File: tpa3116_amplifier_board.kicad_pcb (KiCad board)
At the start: 2 copper layers, 61.6 x 50.8 mm, 41 parts, among them IC1 TPA3116D2QDADRQ1, J1 power_supply, J2 Conn_01x04, J3 power_supply, J4 output_right

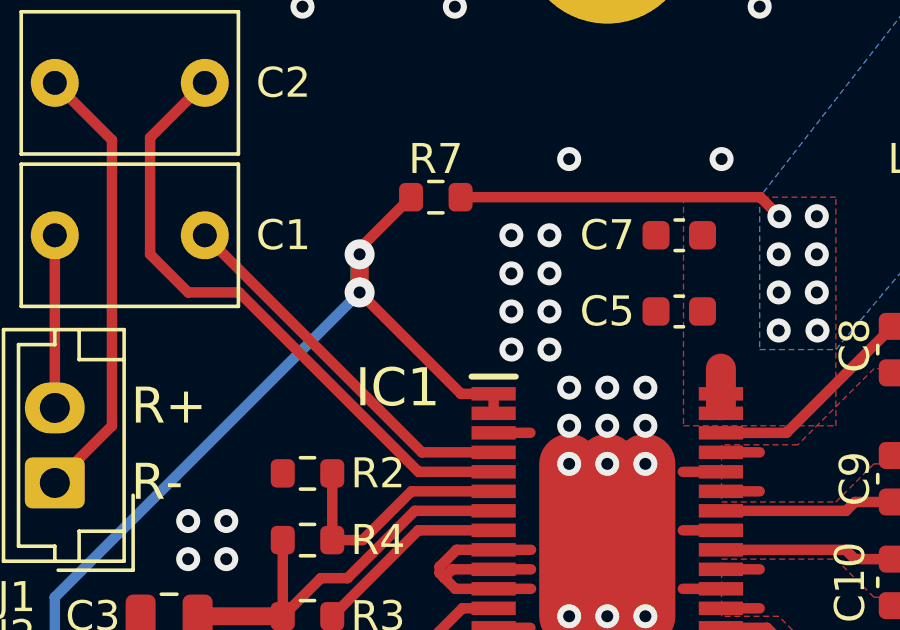
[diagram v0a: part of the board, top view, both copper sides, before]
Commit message: исправил ошибку в схеме
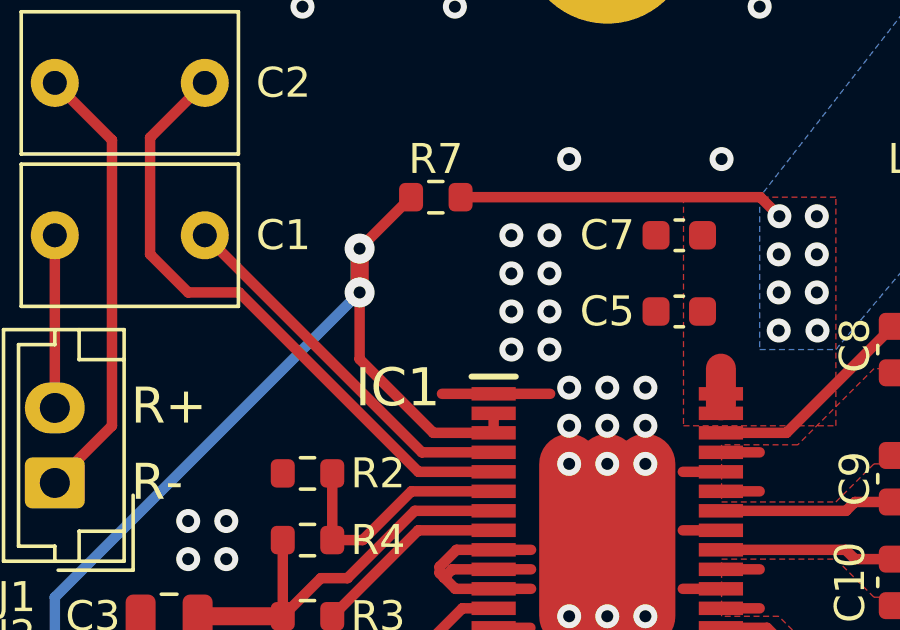
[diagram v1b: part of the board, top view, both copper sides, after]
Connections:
- IC1 pad 1: /SD_LR -> GND
- IC1 pad 3: GND -> /SD_LR
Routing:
- net GND: track 38.0 -> 40.4 mm
- net /SD_LR: track 31.2 -> 33.2 mm
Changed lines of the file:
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@@
       (stroke (width 0.1) (type solid)) (layer "F.Fab"))
     (pad "1" smd rect (at -3.788 -4.875 90) (size 0.45 1.475) (layers "F.Cu" "F.Paste" "F.Mask")
-      (net 16 "/SD_LR") (pinfunction "MODSEL") (pintype "passive"))
+      (net 5 "GND") (pinfunction "MODSEL") (pintype "passive"))
     (pad "2" smd rect (at -3.788 -4.225 90) (size 0.45 1.475) (layers "F.Cu" "F.Paste" "F.Mask")
       (net 16 "/SD_LR") (pinfunction "SD") (pintype "passive"))
     (pad "3" smd rect (at -3.788 -3.575 90) (size 0.45 1.475) (layers "F.Cu" "F.Paste" "F.Mask")
-      (net 5 "GND") (pinfunction "FAULT") (pintype "passive"))
+      (net 16 "/SD_LR") (pinfunction "FAULT") (pintype "passive"))
     (pad "4" smd rect (at -3.788 -2.925 90) (size 0.45 1.475) (layers "F.Cu" "F.Paste" "F.Mask")
       (net 2 "Net-(IC1-RINP)") (pinfunction "RINP") (pintype "passive"))
@@
   (segment (start 128.248 121.64) (end 126.978 121.64) (width 0.35) (layer "F.Cu") (net 5))
   (segment (start 120.672 124.24) (end 121.898 124.24) (width 0.35) (layer "F.Cu") (net 5))
-  (segment (start 120.672 116.44) (end 121.898 116.44) (width 0.35) (layer "F.Cu") (net 5))
   (segment (start 120.672 121.64) (end 121.92 121.64) (width 0.35) (layer "F.Cu") (net 5))
   (segment (start 120.672 120.34) (end 121.92 120.34) (width 0.35) (layer "F.Cu") (net 5))
   (segment (start 128.248 117.74) (end 126.978 117.74) (width 0.35) (layer "F.Cu") (net 5))
+  (segment (start 122.555 115.14) (end 118.95 115.14) (width 0.35) (layer "F.Cu") (net 5))
   (segment (start 119.294 120.99) (end 120.672 120.99) (width 0.35) (layer "F.Cu") (net 5))
   (segment (start 120.672 123.59) (end 121.898 123.59) (width 0.35) (layer "F.Cu") (net 5))
@@
   (segment (start 129.785 122.94) (end 133.985 127.14) (width 0.35) (layer "F.Cu") (net 15))
   (segment (start 128.248 122.94) (end 129.785 122.94) (width 0.35) (layer "F.Cu") (net 15))
-  (segment (start 119.585 115.14) (end 120.672 115.14) (width 0.35) (layer "F.Cu") (net 16))
-  (segment (start 116.205 110.3) (end 116.205 110.49) (width 0.35) (layer "F.Cu") (net 16))
-  (segment (start 120.672 115.79) (end 120.672 115.14) (width 0.35) (layer "F.Cu") (net 16))
-  (segment (start 116.205 111.76) (end 119.585 115.14) (width 0.35) (layer "F.Cu") (net 16))
-  (segment (start 116.205 110.49) (end 116.205 111.76) (width 0.6) (layer "F.Cu") (net 16))
-  (segment (start 117.92 108.585) (end 116.205 110.3) (width 0.35) (layer "F.Cu") (net 16))
-  (via (at 116.205 110.49) (size 1) (drill 0.4) (layers "F.Cu" "B.Cu") (net 16))
+  (segment (start 118.6625 116.44) (end 120.672 116.44) (width 0.35) (layer "F.Cu") (net 16))
+  (segment (start 116.205 110.3) (end 117.92 108.585) (width 0.35) (layer "F.Cu") (net 16))
+  (segment (start 120.672 116.44) (end 120.672 115.79) (width 0.35) (layer "F.Cu") (net 16))
+  (segment (start 116.205 111.76) (end 116.205 113.9825) (width 0.35) (layer "F.Cu") (net 16))
+  (segment (start 116.205 113.9825) (end 118.6625 116.44) (width 0.35) (layer "F.Cu") (net 16))
+  (segment (start 116.205 110.3) (end 116.205 111.76) (width 0.6) (layer "F.Cu") (net 16))
+  (via (at 116.205 110.3) (size 1) (drill 0.4) (layers "F.Cu" "B.Cu") (net 16))
   (via (at 116.205 111.76) (size 1) (drill 0.4) (layers "F.Cu" "B.Cu") (net 16))
+  (segment (start 106.045 121.92) (end 106.045 127.04) (width 0.35) (layer "B.Cu") (net 16))
+  (segment (start 116.205 110.3) (end 116.205 111.76) (width 0.6) (layer "B.Cu") (net 16))
   (segment (start 116.205 111.76) (end 106.045 121.92) (width 0.35) (layer "B.Cu") (net 16))
-  (segment (start 116.205 110.49) (end 116.205 111.76) (width 0.6) (layer "B.Cu") (net 16))
-  (segment (start 106.045 121.92) (end 106.045 127.04) (width 0.35) (layer "B.Cu") (net 16))
   (segment (start 115.293 124.7775) (end 115.293 122.555) (width 0.35) (layer "F.Cu") (net 17))
   (segment (start 120.672 119.69) (end 118.158 119.69) (width 0.35) (layer "F.Cu") (net 17))
